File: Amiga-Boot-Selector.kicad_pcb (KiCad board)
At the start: 2 copper layers, 20.6 x 57.4 mm, 7 parts, among them J1 Conn_01x02, U1 CIA8520 socket, U2 74LS153, U3 CIA8520 pin header

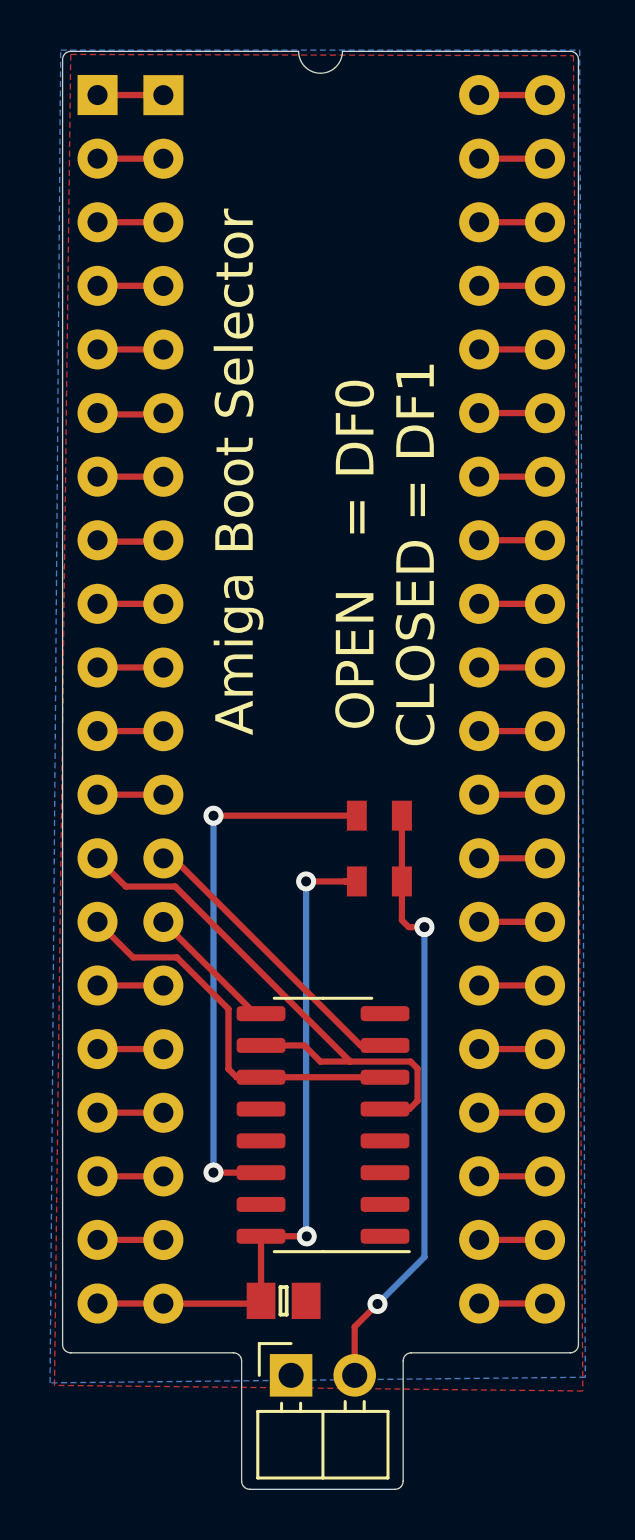
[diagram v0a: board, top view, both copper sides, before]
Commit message: saved
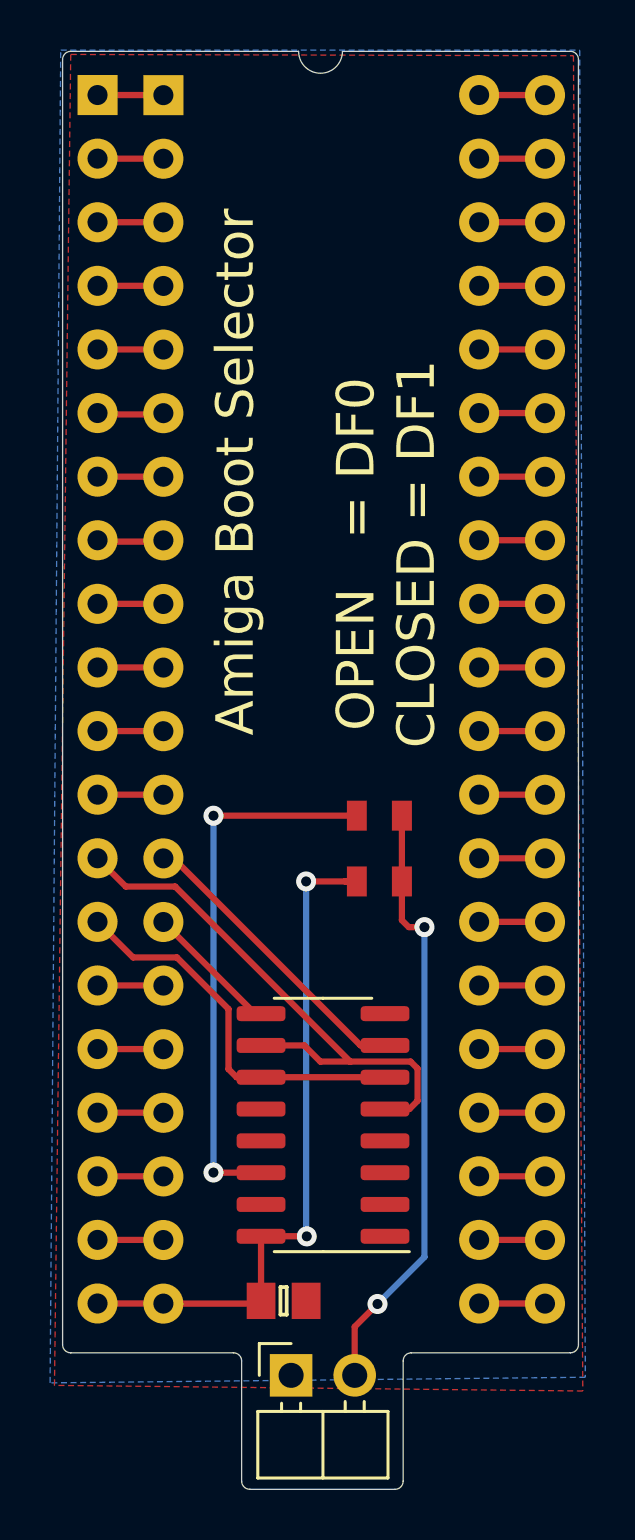
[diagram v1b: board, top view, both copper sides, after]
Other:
- outline, holes or cut-outs redrawn
- net class Default removed
